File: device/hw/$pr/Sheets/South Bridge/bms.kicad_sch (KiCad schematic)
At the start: 32 parts, among them U1 BQ27441DRZR-G1B, U2 BQ24074RGTR, U3 TPS63020DSJR

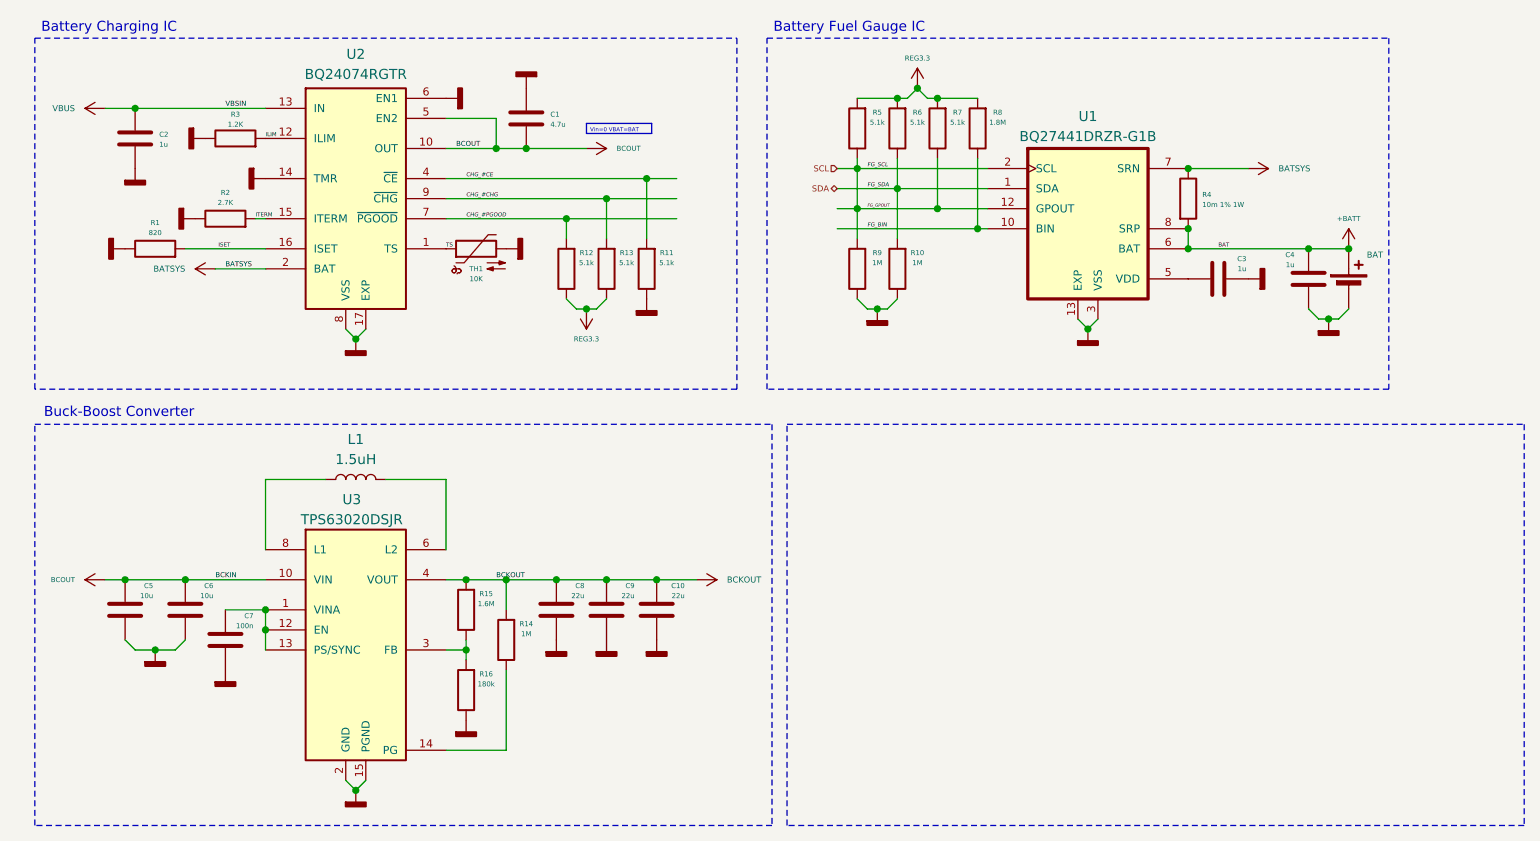
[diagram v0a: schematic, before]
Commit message: application
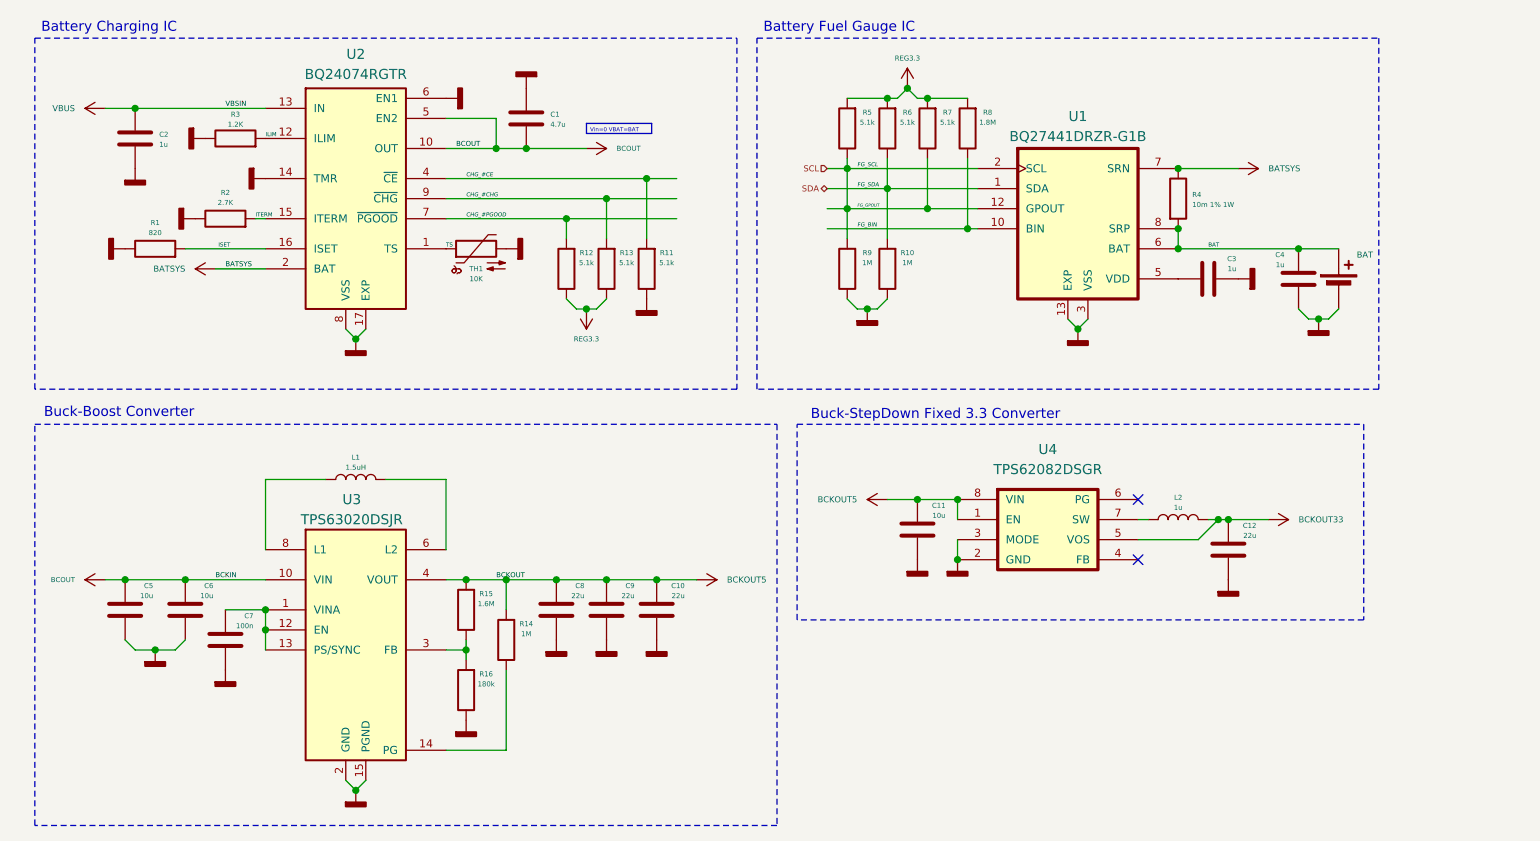
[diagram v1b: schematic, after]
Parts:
- added C11: 10u, symbol Device:C
- added C12: 22u, symbol Device:C
- added L2: 1u, symbol Device:L
- added U4: TPS62082DSGR, fpl:TPS62082DSGR, symbol syl:TPS62082DSGR
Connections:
- net +BATT renamed BAT
- net BCKOUT renamed BCKOUT5
- net BCKOUT5: now also C11.2, U4.1 (EN), U4.8 (VIN)
- net GNDD renamed GND
- net GND: now also C11.1, C12.1, U4.2 (GND), U4.3 (MODE), U4.9 (GND), U4.9_1 (GND), U4.9_2 (GND)
- new net: L2.1, U4.7 (SW)
- new net BCKOUT33: C12.2, L2.2, U4.5 (VOS)
- no-connect marks 0 -> 2
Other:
- note added: "Buck-StepDown Fixed 3.3 Converter"
- moved on the sheet: BAT, C3, C4, R10, R4, R5, R6, R7, R8, R9, U1
